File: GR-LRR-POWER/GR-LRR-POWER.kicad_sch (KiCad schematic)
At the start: 44 parts, among them J1 DT13-08PB, J2 DT13-08PB, J3 691137710002, U1 SIS434DN-T1-GE3, U2 SIS434DN-T1-GE3, U3 LTC4365CTS8-TRMPBF, U5 696108003002, U6 696108003002, U7 696108003002

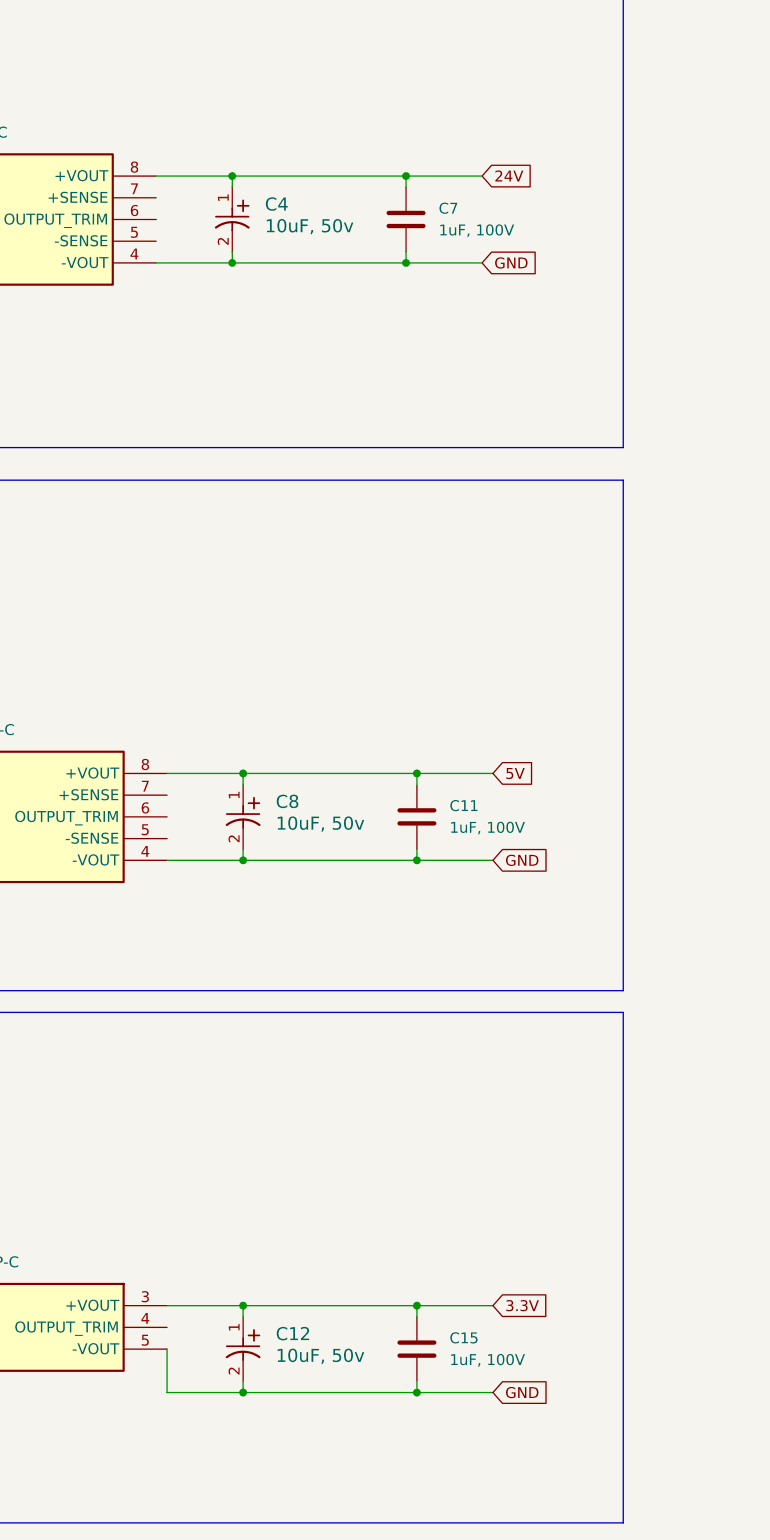
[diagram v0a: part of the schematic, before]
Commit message: ordered power and control A4
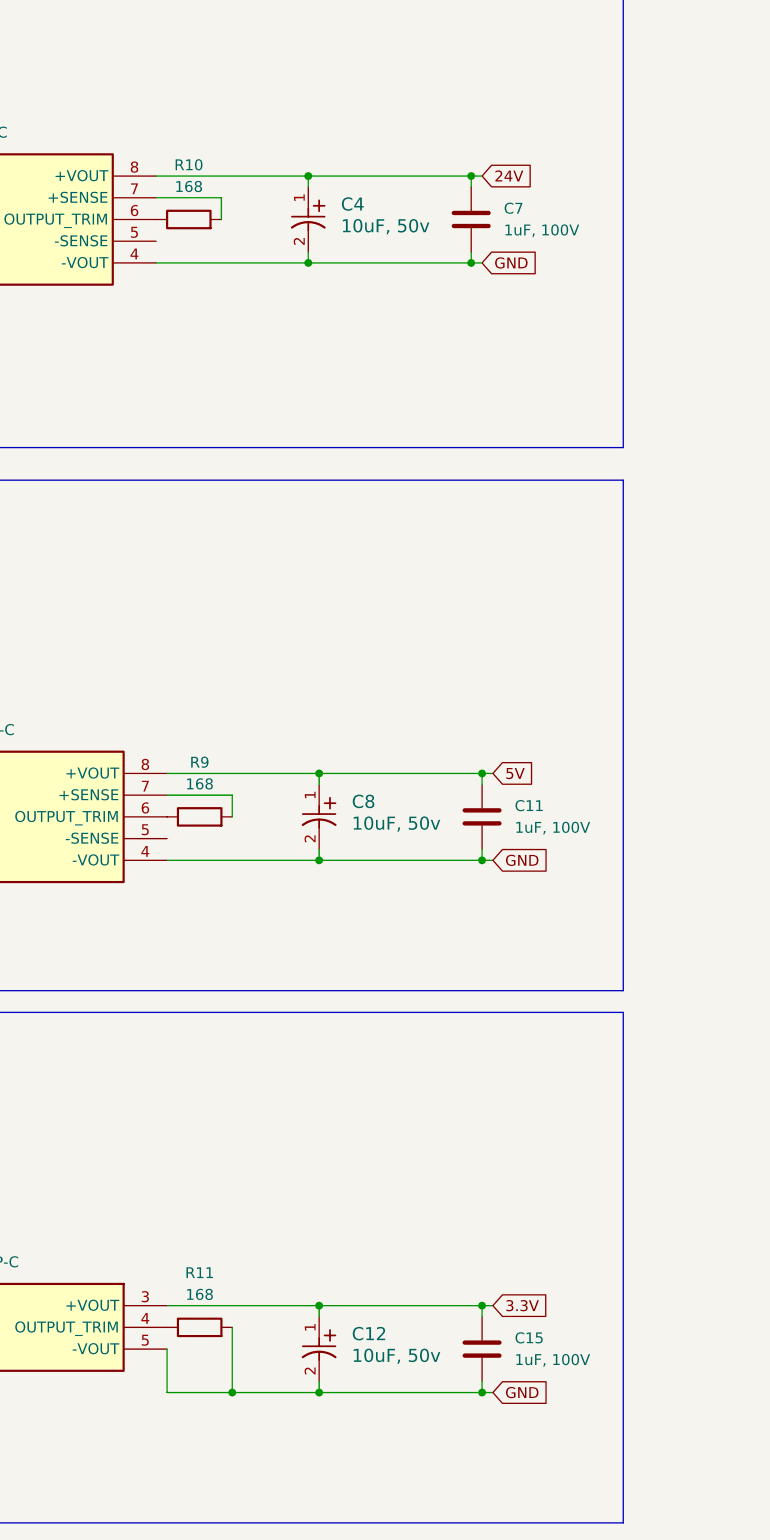
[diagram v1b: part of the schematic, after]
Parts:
- added R10, R11, R9: 168, Resistor_SMD:R_1206_3216Metric_Pad1.30x1.75mm_HandSolder, symbol Device:R
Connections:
- net GND: now also R11.2
- net at PS3.4 (OUTPUT_TRIM): now also R11.1
- net at PS1.6 (OUTPUT_TRIM): now also R10.1
- net at PS1.7 (+SENSE): now also R10.2
- net at PS2.6 (OUTPUT_TRIM): now also R9.1
- net at PS2.7 (+SENSE): now also R9.2
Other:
- moved on the sheet: C11, C12, C15, C4, C7, C8
